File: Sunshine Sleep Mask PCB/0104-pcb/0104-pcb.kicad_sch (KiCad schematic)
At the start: 8 parts, among them J1 Conn_01x02, J2 Conn_01x02, J3 Conn_01x04, J5 Conn_01x15, J6 Conn_01x15, U3 MAX98357A

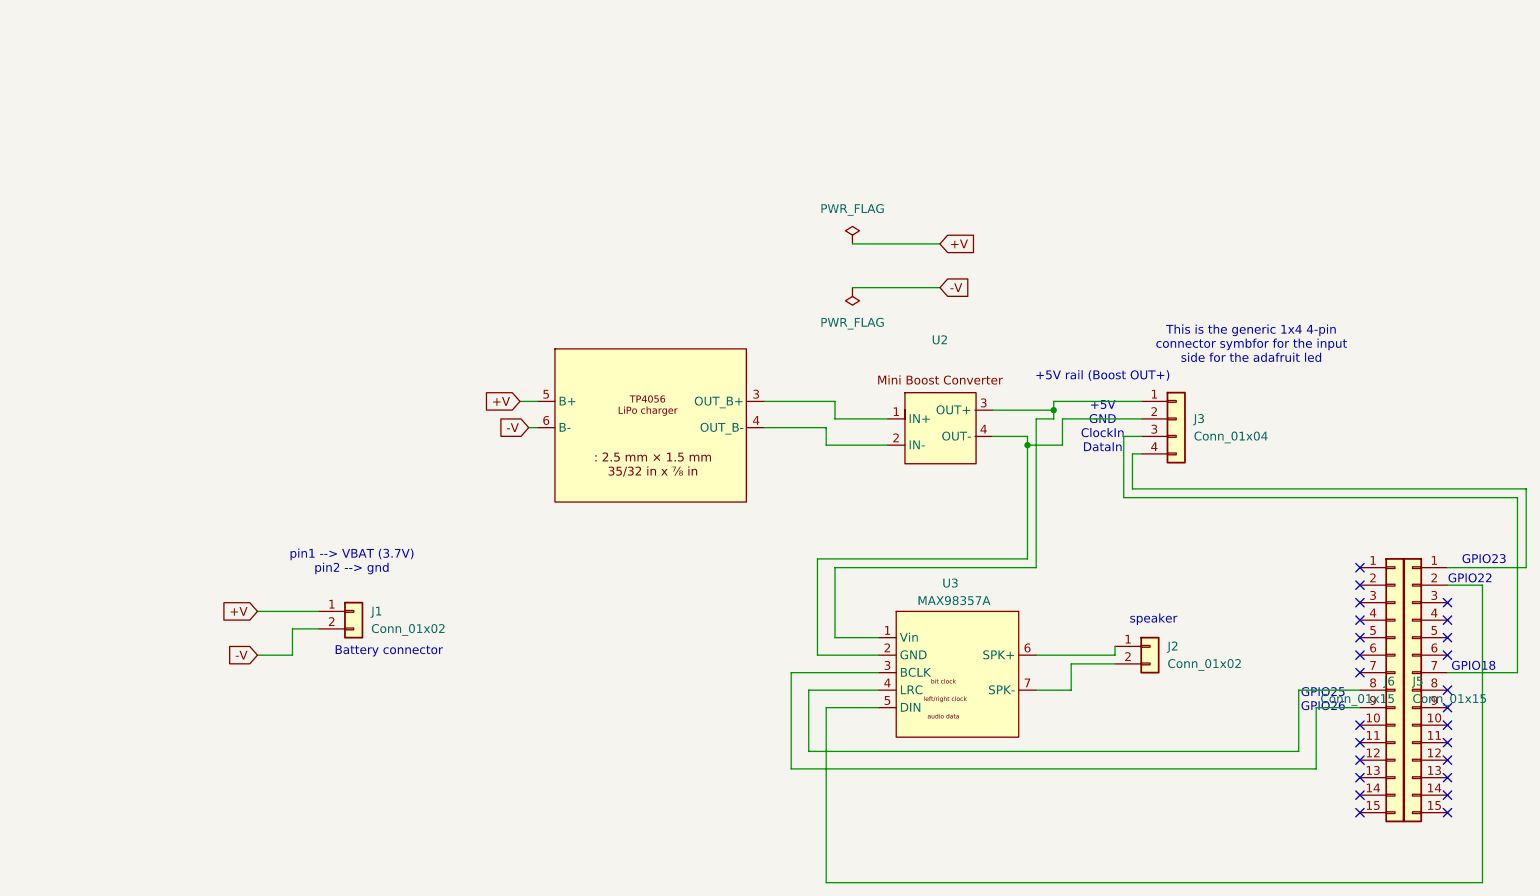
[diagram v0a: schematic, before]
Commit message: Clay 0408 Changes
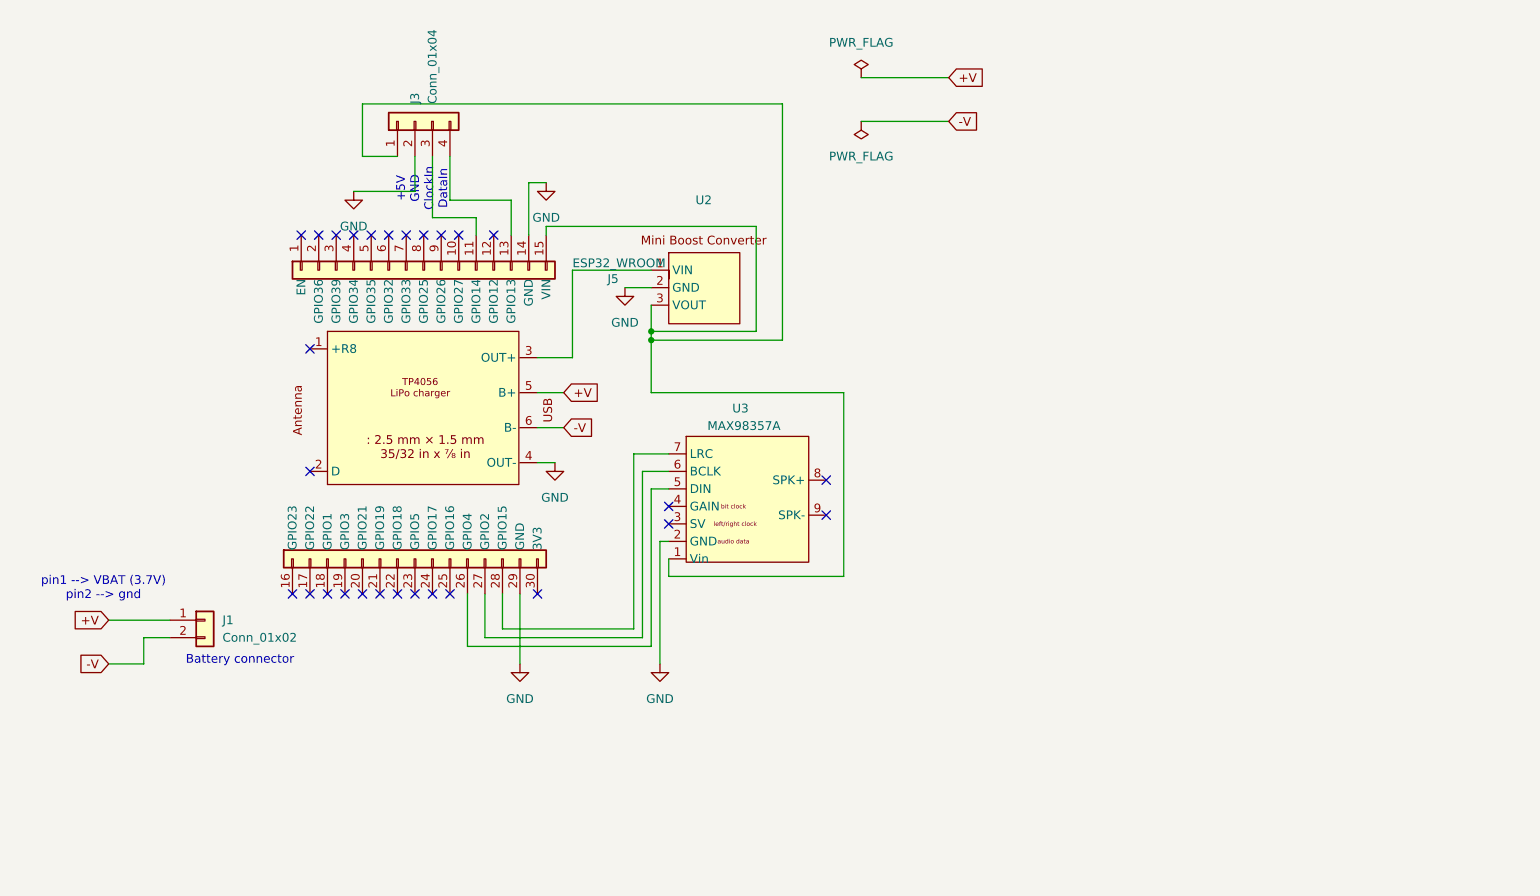
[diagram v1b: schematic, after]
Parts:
- removed J2: Conn_01x02, Connector_PinHeader_2.54mm:PinHeader_1x02_P2.54mm_Vertical, symbol Connector_Generic:Conn_01x02
- removed J6: Conn_01x15, Connector_PinSocket_2.54mm:PinSocket_1x15_P2.54mm_Vertical, symbol Connector_Generic:Conn_01x15
- J5: value Conn_01x15 -> ESP32_WROOM; footprint Connector_PinSocket_2.54mm:PinSocket_1x15_P2.54mm_Vertical -> RF_Module:ESP32_WROOM_DevKit_30Pin_Custom
- U2: footprint Library_customized_0104:boost_converter -> Library_customized_0104:Boost_Converter_Clay_Custom
- U3: footprint Library_customized_0104:amplifier_github -> Library_customized_0104:adafruit-MAX98357
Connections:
- net at J3.1 (Pin_1), U2.3 (VOUT), U3.1 (Vin): now also J5.15 (VIN)
- net GND: now reaches J3.2 (Pin_2), U3.2 (GND)
- net GND: now also J5.14 (GND), J5.29 (GND), U1.4 (OUT-), U2.2 (GND); no longer U2.4 (OUT-)
- net at U3.3 (SV): no longer J5.9 (Pin_9)
- net at U3.4 (GAIN): no longer J5.8 (Pin_8)
- net at U3.5 (DIN): now also J5.26 (GPIO4)
- net at U3.6 (BCLK): now also J5.27 (GPIO2)
- net at U3.7 (LRC): now also J5.28 (GPIO15)
- net at J3.3 (Pin_3): now also J5.11 (GPIO14)
- net at J3.4 (Pin_4): now also J5.13 (GPIO13)
- no-connect marks 25 -> 28
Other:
- note removed: "+5V rail (Boost OUT+)"
- note removed: "GPIO18"
- note removed: "GPIO22"
- note removed: "GPIO23"
- note removed: "GPIO25"
- note removed: "GPIO26"
- note removed: "This is the generic 1x4 4-pin connector symbfor for the input side for the adafruit led"
- note removed: "speaker"
- moved on the sheet: J1, J3
